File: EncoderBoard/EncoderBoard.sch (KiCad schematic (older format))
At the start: 40 parts, among them U1 MCP23S17_SO, U2 MCP23S17_SO, U3 MCP23S17_SO, U4 TCA9548APWR, U5 74HCT245, U6 TCA9548APWR, U7 Teensy3.2, U8 CAT24M01W

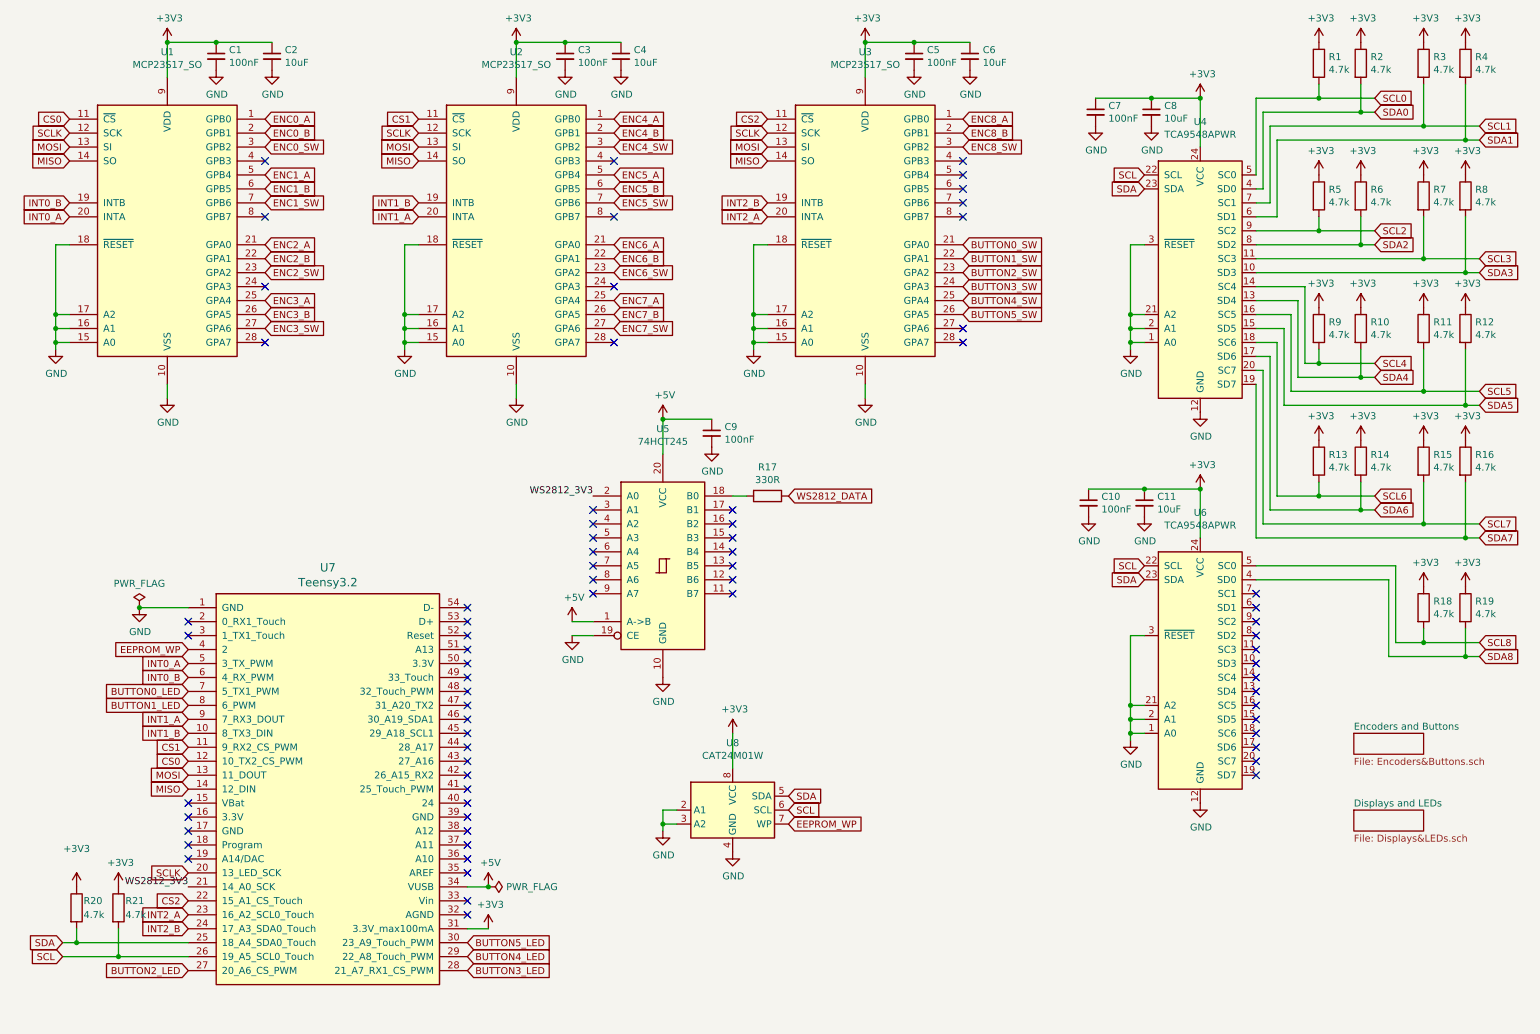
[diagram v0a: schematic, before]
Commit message: Tidied up the encoder board, updated debounce logic for schematic.
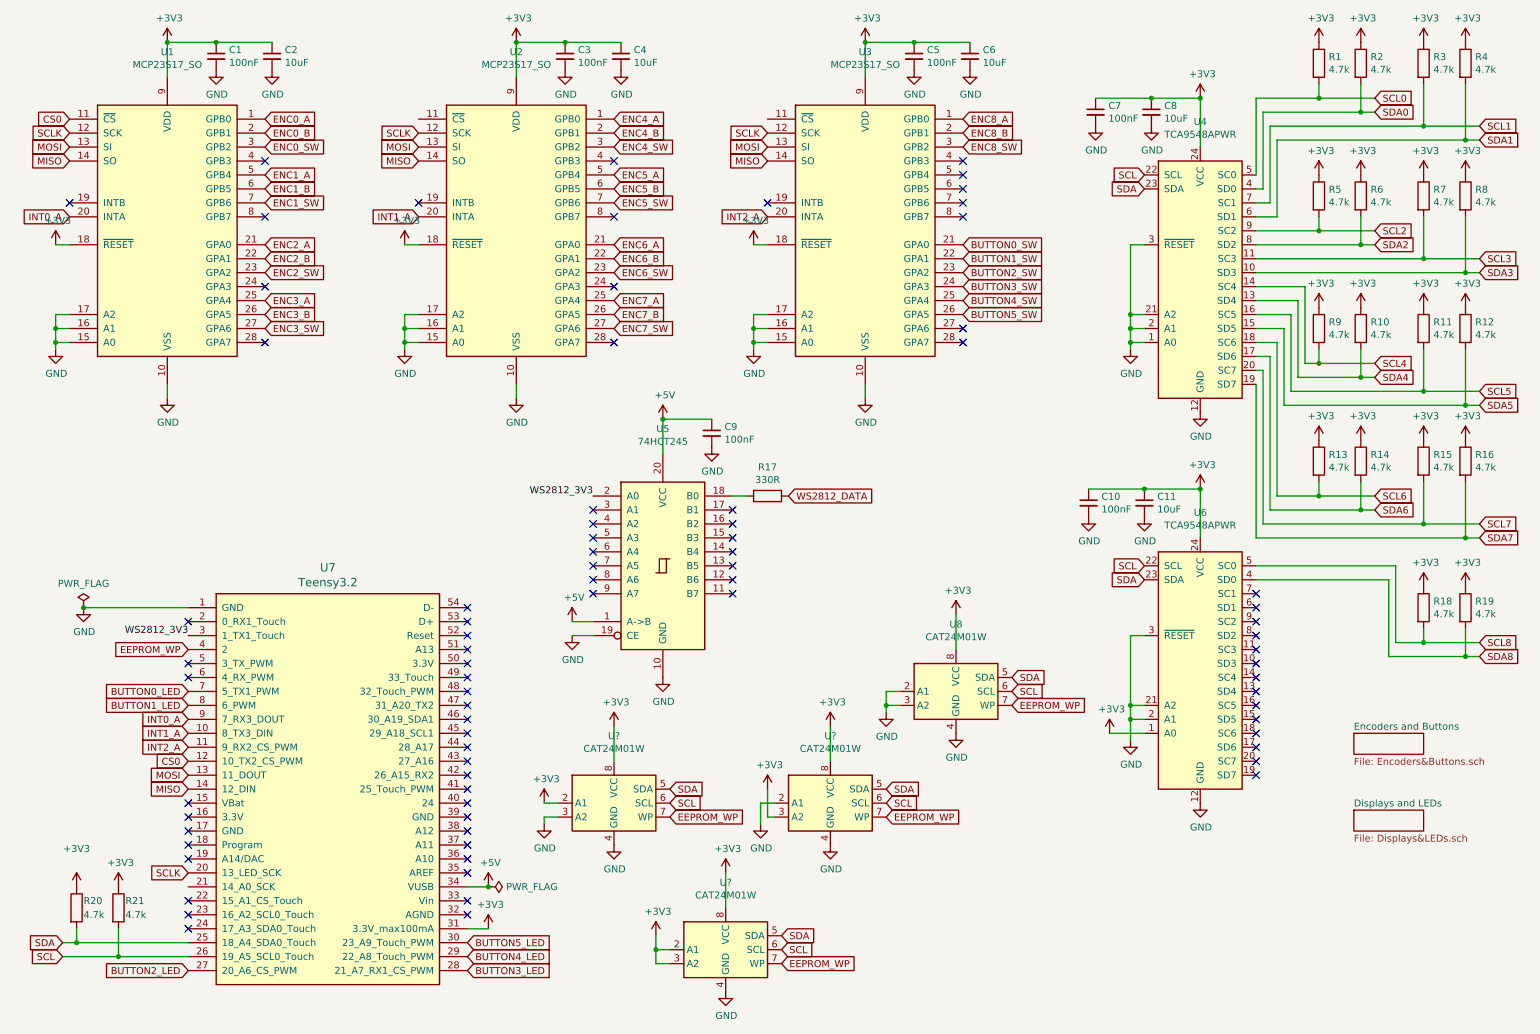
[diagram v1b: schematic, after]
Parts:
- added U? (x3): CAT24M01W, SOIC_BG:SOIC-8_3.9x4.9mm_P1.27mm, symbol Memory_EEPROM:CAT24M01W
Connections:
- net +3V3: now also U1.18 (~RESET~), U2.18 (~RESET~), U3.18 (~RESET~), U6.1 (A0), U?.2 (A1), U?.2 (A1), U?.3 (A2), U?.3 (A2), U?.8 (VCC), U?.8 (VCC), U?.8 (VCC)
- net EEPROM_WP: now also U?.7 (WP), U?.7 (WP), U?.7 (WP)
- net GND: now also U?.2 (A1), U?.3 (A2), U?.4 (GND), U?.4 (GND), U?.4 (GND); no longer U1.18 (~RESET~), U2.18 (~RESET~), U3.18 (~RESET~), U6.1 (A0)
- net INT0_A: now also U7.9 (7_RX3_DOUT); no longer U7.5 (3_TX_PWM)
- net INT1_A: now also U7.10 (8_TX3_DIN); no longer U7.9 (7_RX3_DOUT)
- net INT2_A: now also U7.11 (9_RX2_CS_PWM); no longer U7.23 (16_A2_SCL0_Touch)
- net SCL: now also U?.6 (SCL), U?.6 (SCL), U?.6 (SCL)
- net SDA: now also U?.5 (SDA), U?.5 (SDA), U?.5 (SDA)
- net WS2812_3V3: now also U7.3 (1_TX1_Touch); no longer U7.21 (14_A0_SCK)
- net CS1: no longer names the net of U2.11 (~CS~)
- net CS1: no longer U7.11 (9_RX2_CS_PWM)
- net CS2: no longer names the net of U7.22 (15_A1_CS_Touch)
- net CS2: no longer U3.11 (~CS~)
- net INT0_B: no longer names the net of U7.6 (4_RX_PWM)
- net INT0_B: no longer U1.19 (INTB)
- net INT1_B: no longer names the net of U2.19 (INTB)
- net INT1_B: no longer U7.10 (8_TX3_DIN)
- net INT2_B: no longer names the net of U7.24 (17_A3_SDA0_Touch)
- net INT2_B: no longer U3.19 (INTB)
- no-connect marks 72 -> 79
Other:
- moved on the sheet: U8
